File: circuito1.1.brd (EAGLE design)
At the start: 57.5 x 83.9 mm, 40 parts

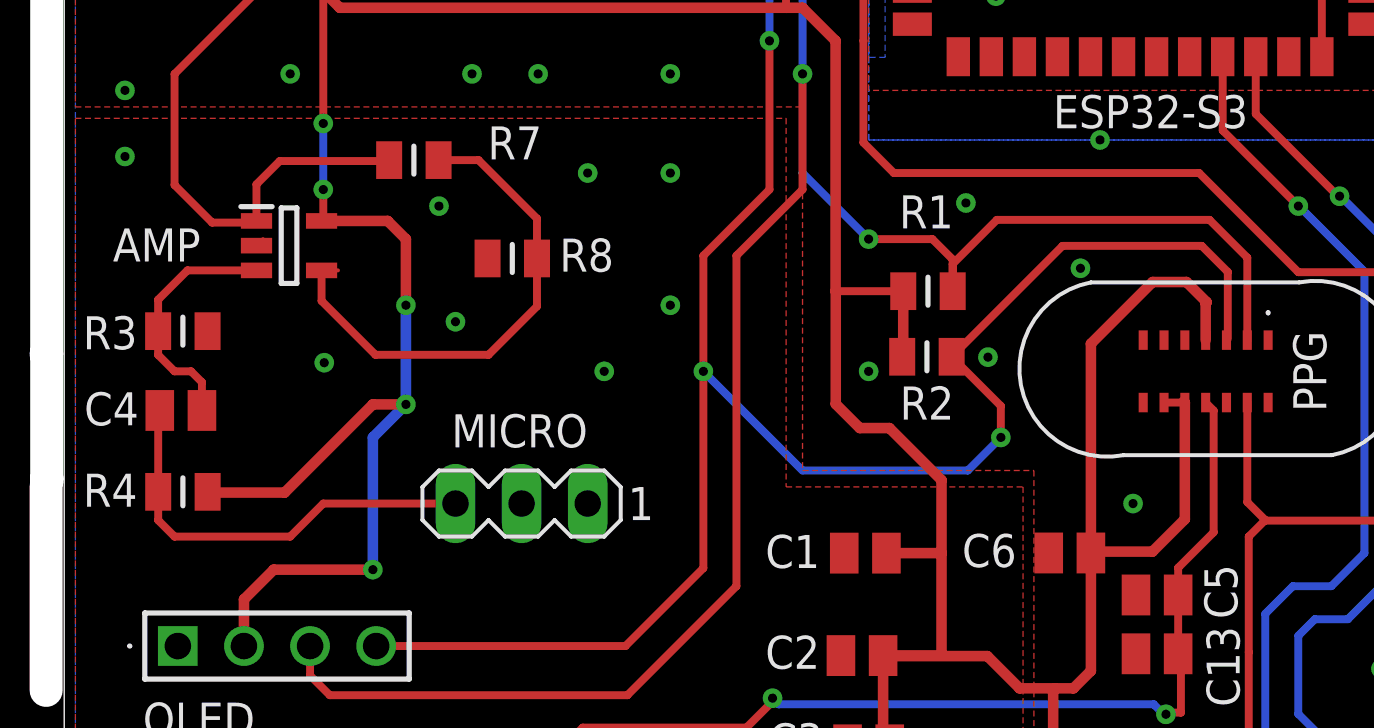
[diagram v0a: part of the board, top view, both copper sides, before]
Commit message: ultima revision
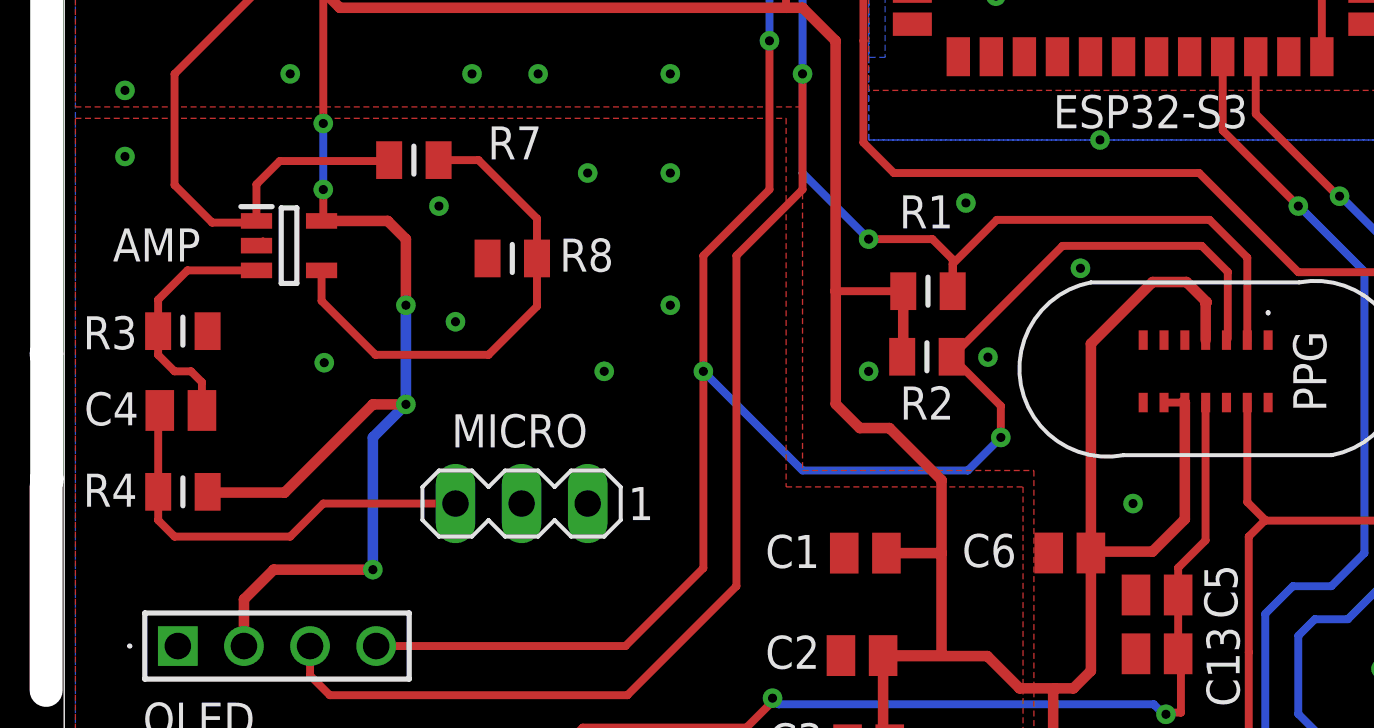
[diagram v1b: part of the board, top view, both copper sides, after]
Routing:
- net N$1: track 10.4 -> 9.57 mm
- net N$4: track 21.1 -> 20.5 mm
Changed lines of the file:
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@@
 <wire x1="58.559" y1="48.756" x2="58.406" y2="48.756" width="0.1524" layer="1"/>
 <wire x1="53.978" y1="44.45" x2="53.909" y2="44.519" width="0.1524" layer="1"/>
-<wire x1="53.909" y1="44.519" x2="54.541" y2="44.519" width="0.1524" layer="1"/>
 <wire x1="62.23" y1="44.935" x2="62.187" y2="44.978" width="0.1524" layer="1"/>
 <wire x1="53.909" y1="44.519" x2="53.909" y2="43.346290625" width="0.3048" layer="1"/>
@@
 <contactref element="C4" pad="2"/>
 <contactref element="AMP" pad="3"/>
-<wire x1="47.6295" y1="43.0575" x2="47.6295" y2="42.1845" width="0.1524" layer="1"/>
 <wire x1="47.6295" y1="42.1845" x2="47.6295" y2="43.3930625" width="0.3048" layer="1"/>
 <wire x1="48.7554375" y1="44.519" x2="51.409" y2="44.519" width="0.3048" layer="1"/>
@@
 <contactref element="AMP" pad="1"/>
 <contactref element="R7" pad="1"/>
-<wire x1="56.515" y1="48.765" x2="56.506" y2="48.756" width="0.1524" layer="1"/>
 <wire x1="48.26" y1="52.0653375" x2="52.07" y2="55.8753375" width="0.3048" layer="1"/>
 <wire x1="48.26" y1="47.800234375" x2="48.26" y2="52.0653375" width="0.3048" layer="1"/>
@@
 <wire x1="51.409" y1="46.419" x2="51.345" y2="46.355" width="0.3048" layer="1"/>
 <wire x1="51.345" y1="46.355" x2="49.705234375" y2="46.355" width="0.3048" layer="1"/>
-<wire x1="56.506" y1="48.756" x2="56.47076875" y2="48.72076875" width="0.3048" layer="1"/>
 <wire x1="52.3028625" y1="48.72076875" x2="51.407340625" y2="47.825246875" width="0.3048" layer="1"/>
 <wire x1="51.407340625" y1="47.825246875" x2="51.407340625" y2="46.420659375" width="0.3048" layer="1"/>
 <wire x1="51.407340625" y1="46.420659375" x2="51.409" y2="46.419" width="0.3048" layer="1"/>
 <wire x1="56.47076875" y1="48.72076875" x2="52.3028625" y2="48.72076875" width="0.3048" layer="1"/>
+<wire x1="56.506" y1="48.756" x2="56.515" y2="48.765" width="0.1524" layer="1"/>
+<wire x1="56.506" y1="48.756" x2="56.47076875" y2="48.72076875" width="0.1524" layer="1"/>
 </signal>
 <signal name="TOUCH1">
@@
 <wire x1="86.822953125" y1="29.78683125" x2="86.822953125" y2="32.0469625" width="0.3048" layer="1"/>
 <wire x1="86.822953125" y1="32.0469625" x2="86.822953125" y2="33.091515625" width="0.3048" layer="1"/>
-<wire x1="86.822953125" y1="33.091515625" x2="88.187790625" y2="34.456353125" width="0.3048" layer="1"/>
-<wire x1="88.187790625" y1="34.456353125" x2="88.187790625" y2="39.132209375" width="0.3048" layer="1"/>
-<wire x1="88.187790625" y1="39.132209375" x2="87.88" y2="39.44" width="0.3048" layer="1"/>
+<wire x1="86.822953125" y1="33.091515625" x2="87.876040625" y2="34.144603125" width="0.3048" layer="1"/>
+<wire x1="87.88" y1="39.44" x2="87.876040625" y2="39.436040625" width="0.3048" layer="1"/>
+<wire x1="87.876040625" y1="39.436040625" x2="87.876040625" y2="34.144603125" width="0.3048" layer="1"/>
 <contactref element="REGP" pad="3"/>
 <wire x1="52.1545625" y1="21.709528125" x2="58.703196875" y2="21.709528125" width="0.3048" layer="1"/>

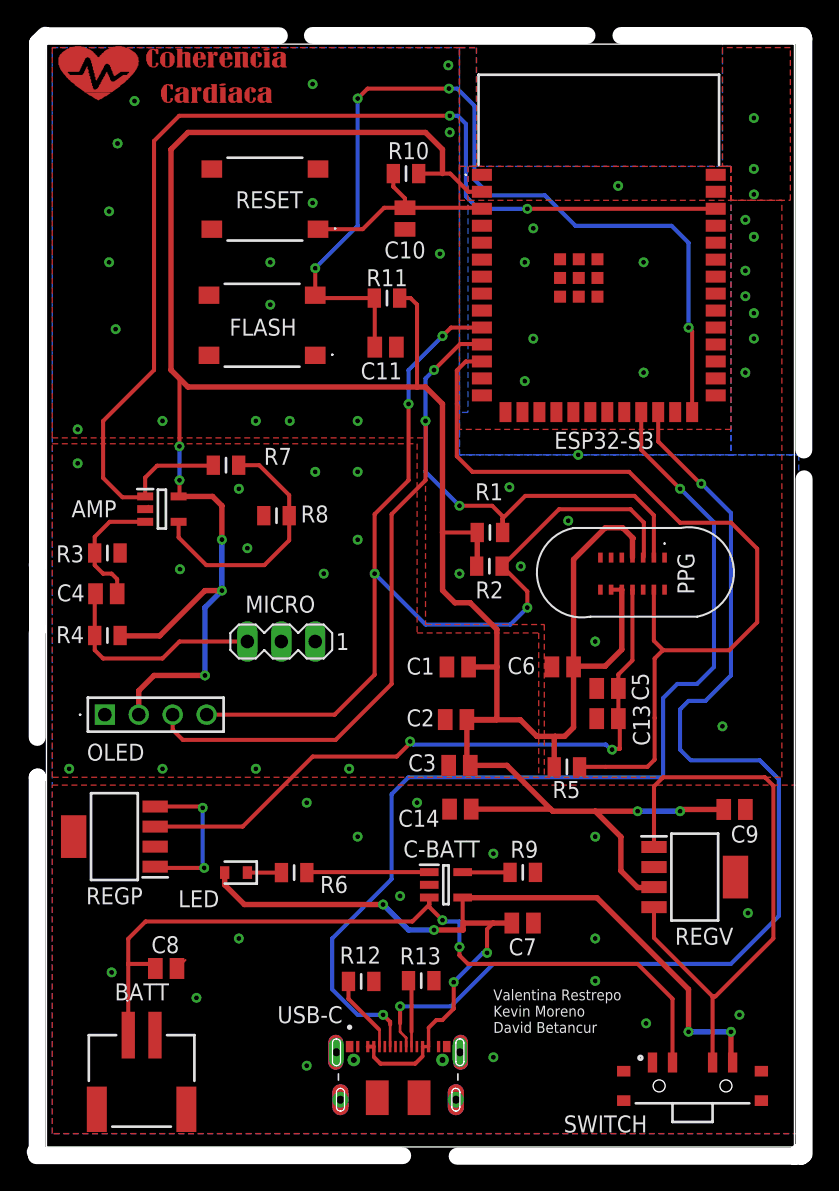
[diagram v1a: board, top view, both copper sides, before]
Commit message: se hicieron correciones que nos dijo el profesor
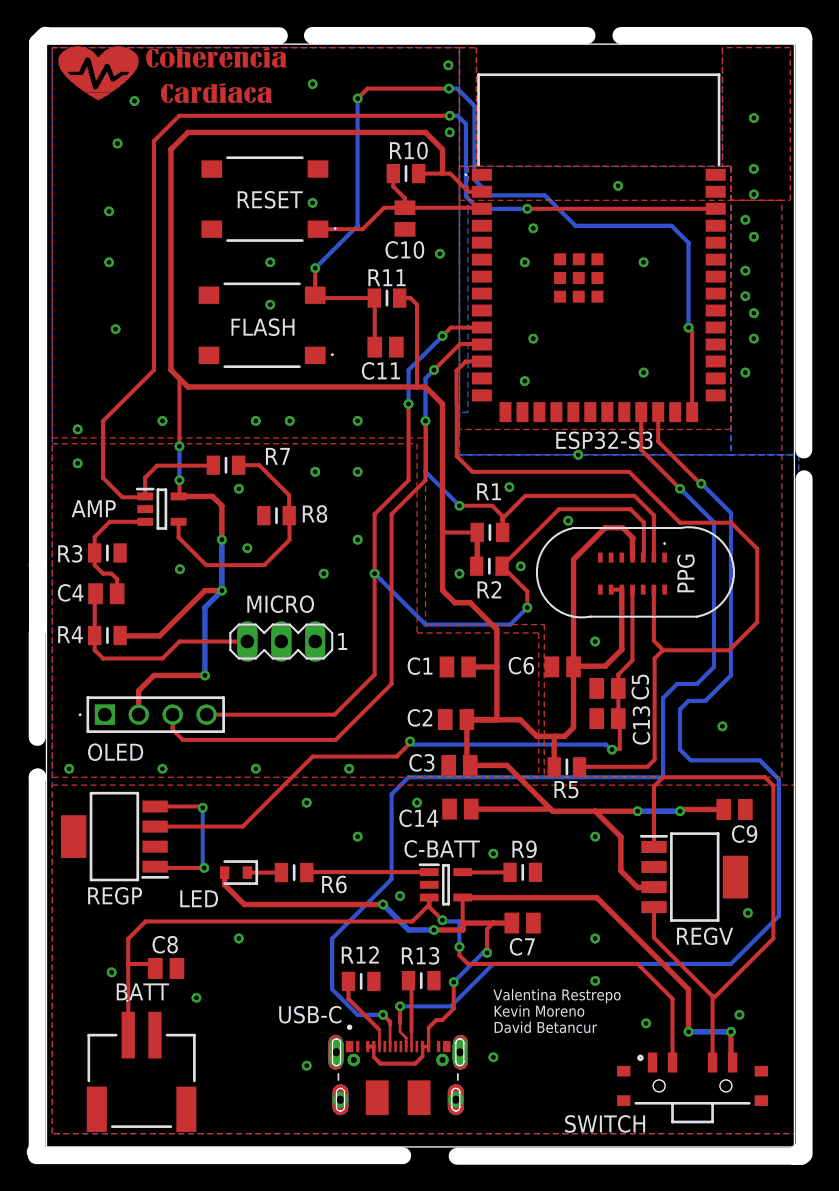
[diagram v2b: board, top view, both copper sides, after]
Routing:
- net N$4: track 20.5 -> 19.4 mm
- net +3V3: track 234.7 -> 234.0 mm
- net N$13: track 4.10 -> 3.55 mm
- net EN: track 16.4 -> 15.9 mm
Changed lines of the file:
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@@
 <contactref element="AMP" pad="4"/>
 <contactref element="R8" pad="2"/>
-<wire x1="62.187" y1="44.45" x2="62.187" y2="44.978" width="0.1524" layer="1"/>
 <wire x1="58.377" y1="48.785" x2="58.406" y2="48.756" width="0.1524" layer="1"/>
-<wire x1="58.406" y1="48.756" x2="58.406" y2="49.163" width="0.1524" layer="1"/>
 <wire x1="58.559" y1="48.756" x2="58.406" y2="48.756" width="0.1524" layer="1"/>
-<wire x1="53.978" y1="44.45" x2="53.909" y2="44.519" width="0.1524" layer="1"/>
-<wire x1="62.23" y1="44.935" x2="62.187" y2="44.978" width="0.1524" layer="1"/>
 <wire x1="53.909" y1="44.519" x2="53.909" y2="43.346290625" width="0.3048" layer="1"/>
 <wire x1="55.980290625" y1="41.275" x2="53.909" y2="43.346290625" width="0.3048" layer="1"/>
 <wire x1="55.980290625" y1="41.275" x2="60.325" y2="41.275" width="0.3048" layer="1"/>
-<wire x1="60.325" y1="41.275" x2="62.187" y2="43.137" width="0.3048" layer="1"/>
-<wire x1="62.187" y1="43.137" x2="62.187" y2="44.978" width="0.3048" layer="1"/>
+<wire x1="60.325" y1="41.275" x2="62.208321875" y2="43.158321875" width="0.3048" layer="1"/>
+<wire x1="62.208321875" y1="44.956678125" x2="62.187" y2="44.978" width="0.3048" layer="1"/>
+<wire x1="62.208321875" y1="44.956678125" x2="62.208321875" y2="43.158321875" width="0.3048" layer="1"/>
 <wire x1="62.187" y1="44.978" x2="62.187" y2="46.510184375" width="0.3048" layer="1"/>
 <wire x1="58.406" y1="48.756" x2="59.941184375" y2="48.756" width="0.3048" layer="1"/>
@@
 <contactref element="C8" pad="2"/>
 <contactref element="R9" pad="2"/>
-<wire x1="53.7885" y1="11.088" x2="54.4235" y2="11.723" width="0.1524" layer="1"/>
+<wire x1="53.7885" y1="11.088" x2="53.7885" y2="11.13064375" width="0.1524" layer="1"/>
+<wire x1="54.188959375" y1="11.531103125" x2="53.7885" y2="11.13064375" width="0.1524" layer="1"/>
 <contactref element="MICRO" pad="2"/>
 <polygon width="0.1524" layer="1" isolate="0.254" orphans="yes">
@@
 <contactref element="R5" pad="1"/>
 <contactref element="ESP32-S3" pad="12"/>
-<wire x1="74.73" y1="53.34" x2="74.73" y2="53.46" width="0.1524" layer="1"/>
+<wire x1="74.73" y1="53.34" x2="74.73" y2="53.438678125" width="0.1524" layer="1"/>
 <wire x1="83.92" y1="26.18" x2="83.64" y2="25.9" width="0.1524" layer="1"/>
-<wire x1="83.64" y1="25.9" x2="83.64" y2="26.37" width="0.1524" layer="1"/>
-<wire x1="74.73" y1="53.34" x2="74.73" y2="55.8459125" width="0.3048" layer="1"/>
+<wire x1="74.708678125" y1="53.361321875" x2="74.708678125" y2="55.824590625" width="0.3048" layer="1"/>
 <wire x1="75.4035875" y1="56.5195" x2="76.6095" y2="56.5195" width="0.3048" layer="1"/>
-<wire x1="74.73" y1="55.8459125" x2="75.4035875" y2="56.5195" width="0.3048" layer="1"/>
+<wire x1="74.708678125" y1="55.824590625" x2="75.4035875" y2="56.5195" width="0.3048" layer="1"/>
 <wire x1="74.73" y1="53.34" x2="74.73" y2="49.4295125" width="0.3048" layer="1"/>
 <wire x1="74.73" y1="49.4295125" x2="75.8995125" y2="48.26" width="0.3048" layer="1"/>
@@
 <wire x1="95.2666625" y1="44.45" x2="97.21430625" y2="42.50235625" width="0.3048" layer="1"/>
 <wire x1="97.21430625" y1="42.50235625" x2="97.21430625" y2="37.00098125" width="0.3048" layer="1"/>
-<wire x1="83.92" y1="26.18" x2="85.87" y2="26.18" width="0.3048" layer="1"/>
 <wire x1="89.48" y1="39.44" x2="89.48" y2="35.615" width="0.3048" layer="1"/>
 <wire x1="89.48" y1="35.615" x2="90.17" y2="34.925" width="0.3048" layer="1"/>
 <wire x1="89.535" y1="34.29" x2="90.148678125" y2="34.903678125" width="0.3048" layer="1"/>
 <wire x1="90.148678125" y1="34.903678125" x2="90.17" y2="34.925" width="0.3048" layer="1"/>
-<wire x1="89.535" y1="29.845" x2="89.535" y2="34.29" width="0.3048" layer="1"/>
+<wire x1="89.535" y1="26.7203875" x2="89.535" y2="34.29" width="0.3048" layer="1"/>
 <wire x1="97.21430625" y1="37.00098125" x2="95.117003125" y2="34.903678125" width="0.3048" layer="1"/>
 <wire x1="95.117003125" y1="34.903678125" x2="90.148678125" y2="34.903678125" width="0.3048" layer="1"/>
-<wire x1="85.87" y1="26.18" x2="88.9946125" y2="26.18" width="0.3048" layer="1"/>
-<wire x1="89.535" y1="26.7203875" x2="89.535" y2="29.845" width="0.3048" layer="1"/>
+<wire x1="83.92" y1="26.18" x2="88.9946125" y2="26.18" width="0.3048" layer="1"/>
 <wire x1="88.9946125" y1="26.18" x2="89.535" y2="26.7203875" width="0.3048" layer="1"/>
+<wire x1="74.73" y1="53.438678125" x2="74.708678125" y2="53.41735625" width="0.1524" layer="1"/>
+<wire x1="74.708678125" y1="53.41735625" x2="74.708678125" y2="53.361321875" width="0.1524" layer="1"/>
 </signal>
 <signal name="N$1">
@@
 <wire x1="94.105" y1="67.945" x2="94.1095" y2="67.9495" width="0.3048" layer="1"/>
 <wire x1="49.705234375" y1="46.355" x2="48.26" y2="47.800234375" width="0.3048" layer="1"/>
-<wire x1="51.409" y1="46.419" x2="51.232" y2="46.419" width="0.3048" layer="1"/>
 <wire x1="51.409" y1="46.419" x2="51.345" y2="46.355" width="0.3048" layer="1"/>
 <wire x1="51.345" y1="46.355" x2="49.705234375" y2="46.355" width="0.3048" layer="1"/>
@@
 <contactref element="ESP32-S3" pad="26"/>
 <contactref element="FLASH" pad="3"/>
-<wire x1="68.402" y1="61.417" x2="68.339" y2="61.48" width="0.1524" layer="1"/>
 <via x="64.135" y="63.5" extent="1-16" drill="0.35"/>
 <wire x1="64.135" y1="63.5" x2="67.31" y2="66.675" width="0.3048" layer="16"/>
@@
 <contactref element="REGV" pad="3"/>
 <wire x1="76.22" y1="41.2" x2="76.1725" y2="41.2475" width="0.1524" layer="1"/>
-<wire x1="76.1725" y1="41.2475" x2="75.96" y2="41.46" width="0.1524" layer="1"/>
 <wire x1="82.02" y1="26.18" x2="82.01" y2="26.18" width="0.4064" layer="1"/>
 <wire x1="82.0897" y1="28.46" x2="82.8" y2="28.46" width="0.4064" layer="1"/>
@@
 <contactref element="C14" pad="2"/>
 <contactref element="PPG" pad="4"/>
-<wire x1="83.193553125" y1="33.383553125" x2="83.47" y2="33.66" width="0.3048" layer="1"/>
 <wire x1="83.47" y1="29.13" x2="83.47" y2="33.66" width="0.4064" layer="1"/>
 <wire x1="82.8" y1="28.46" x2="83.47" y2="29.13" width="0.4064" layer="1"/>
 <wire x1="75.809975" y1="23.01378125" x2="81.76121875" y2="23.01378125" width="0.4064" layer="1"/>
 <wire x1="81.76121875" y1="23.01378125" x2="81.915" y2="22.86" width="0.4064" layer="1"/>
-<wire x1="87.036403125" y1="39.483596875" x2="87.08" y2="39.44" width="0.4064" layer="1"/>
 <wire x1="87.88" y1="41.84" x2="87.88" y2="43.253053125" width="0.4064" layer="1"/>
 <wire x1="87.88" y1="43.253053125" x2="87.91060625" y2="43.283659375" width="0.4064" layer="1"/>
@@
 <contactref element="R9" pad="1"/>
 <contactref element="C-BATT" pad="5"/>
-<wire x1="78.717" y1="18.28143125" x2="78.3345375" y2="17.89896875" width="0.1524" layer="1"/>
 <wire x1="78.717" y1="18.28143125" x2="75.18856875" y2="18.28143125" width="0.3048" layer="1"/>
 <wire x1="75.18856875" y1="18.28143125" x2="75.17" y2="18.3" width="0.3048" layer="1"/>
@@
 <contactref element="C10" pad="1"/>
 <contactref element="RESET" pad="1"/>
-<wire x1="70.484" y1="68.392" x2="70.851" y2="68.025" width="0.1524" layer="1"/>
 <wire x1="76.534" y1="68.025" x2="76.6095" y2="67.9495" width="0.3048" layer="1"/>
 <wire x1="70.851" y1="68.025" x2="76.534" y2="68.025" width="0.3048" layer="1"/>
